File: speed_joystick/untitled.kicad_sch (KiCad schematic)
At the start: 48 parts

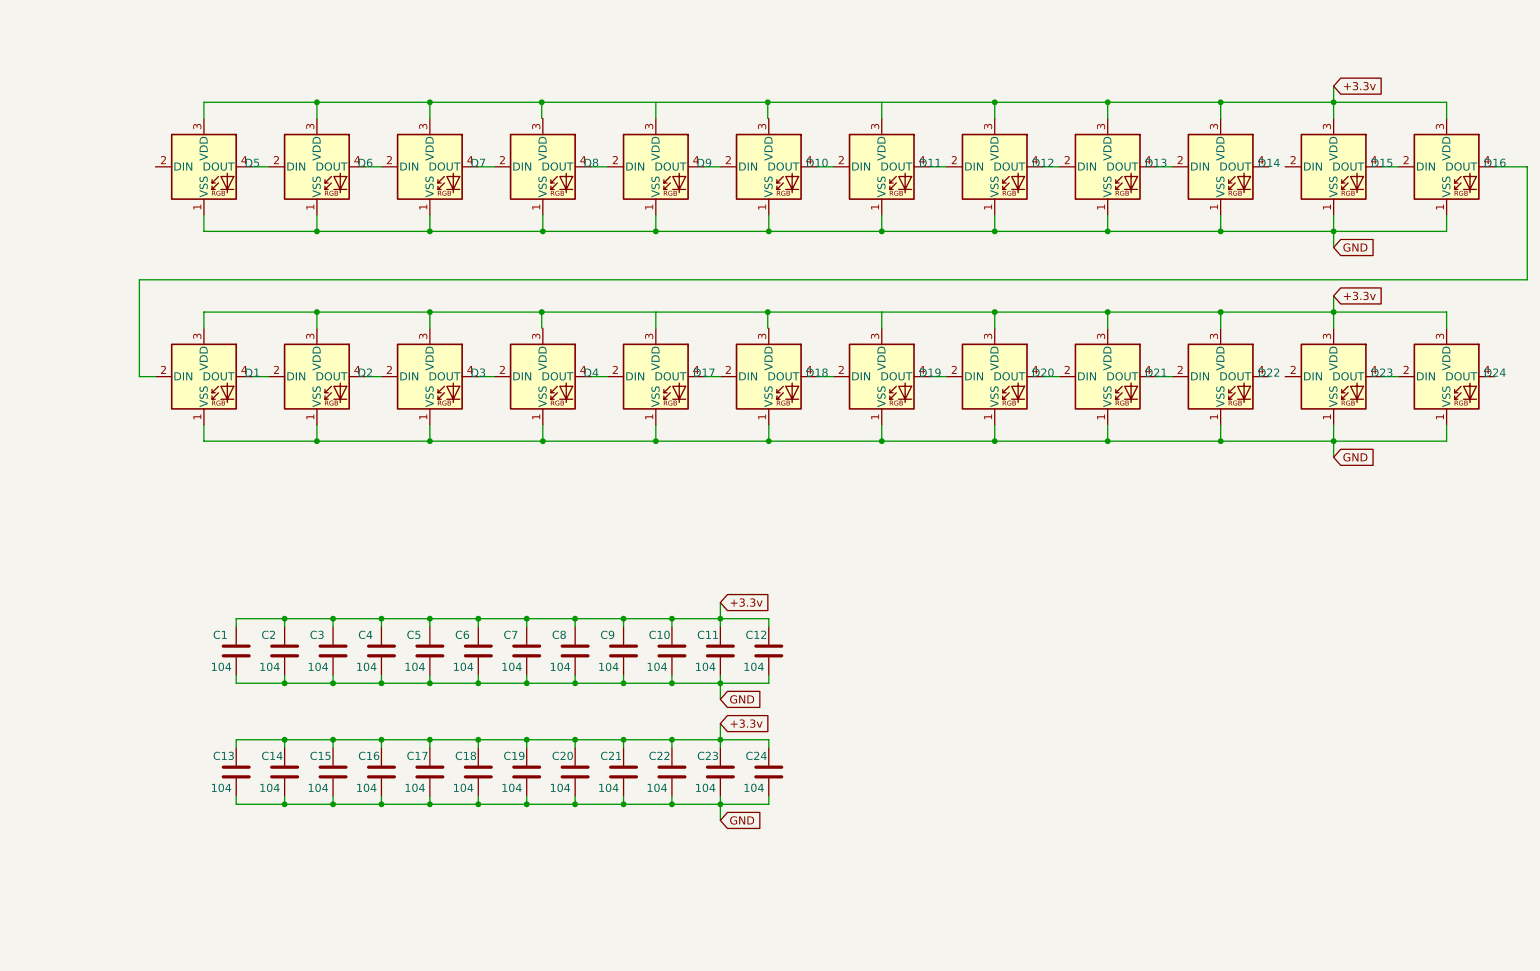
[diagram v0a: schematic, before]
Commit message: work on speed_joystick pcb
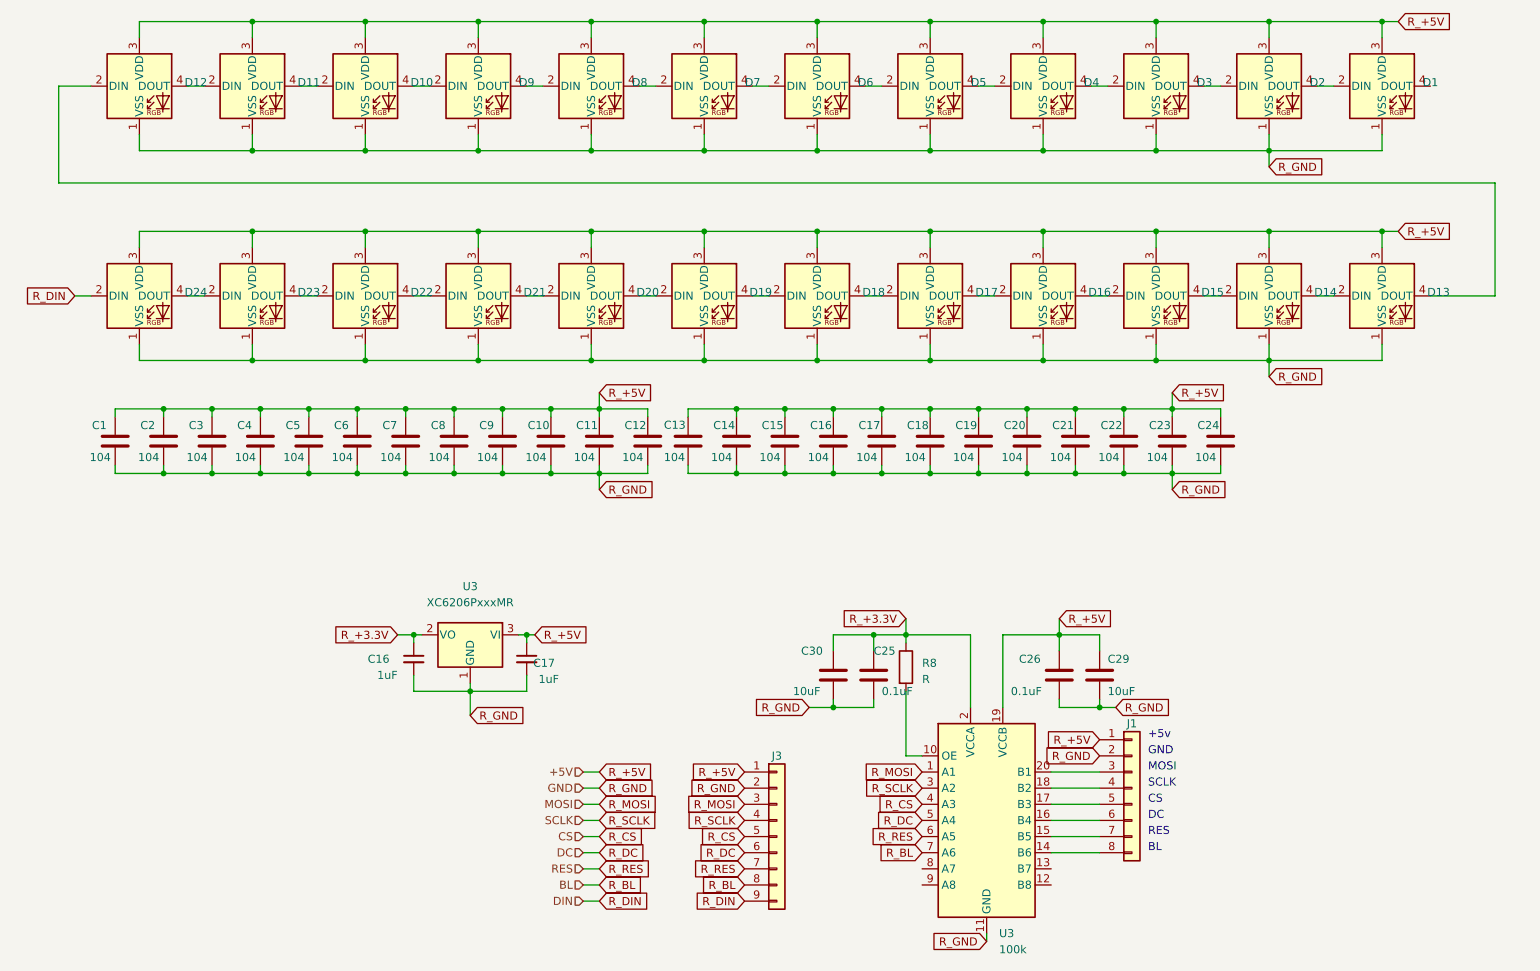
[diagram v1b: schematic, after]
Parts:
- added C16, C17: 1uF, Capacitor_SMD:C_0603_1608Metric, symbol Device:C_Small
- added C25, C26: 0.1uF, Capacitor_SMD:C_0603_1608Metric, symbol Device:C
- added C29, C30: 10uF, Capacitor_SMD:C_0603_1608Metric, symbol Device:C
- added J1: Conn_01x08, 8_hole:8_hole, symbol Connector_Generic:Conn_01x08
- added J3: Conn_01x09, Connector_PinSocket_2.54mm:PinSocket_1x09_P2.54mm_Vertical, symbol Connector_Generic:Conn_01x09
- added R8: R, Resistor_SMD:R_0805_2012Metric, symbol Device:R
- added U3: XC6206PxxxMR, Package_TO_SOT_SMD:SOT-23, symbol Regulator_Linear:XC6206PxxxMR
- added U3: 100k, Package_SO:TSSOP-20_4.4x6.5mm_P0.65mm, symbol Logic_LevelTranslator:TXS0108EPW
- D1: renamed from D16; footprint LED_SMD:LED_SK6812_PLCC4_5.0x5.0mm_P3.2mm -> LED_SMD:my_SK6812
- D10: renamed from D7; footprint LED_SMD:LED_SK6812_PLCC4_5.0x5.0mm_P3.2mm -> LED_SMD:my_SK6812
- D11: renamed from D6; footprint LED_SMD:LED_SK6812_PLCC4_5.0x5.0mm_P3.2mm -> LED_SMD:my_SK6812
- D12: renamed from D5; footprint LED_SMD:LED_SK6812_PLCC4_5.0x5.0mm_P3.2mm -> LED_SMD:my_SK6812
- D13: renamed from D24; footprint LED_SMD:LED_SK6812_PLCC4_5.0x5.0mm_P3.2mm -> LED_SMD:my_SK6812
- D14: renamed from D23; footprint LED_SMD:LED_SK6812_PLCC4_5.0x5.0mm_P3.2mm -> LED_SMD:my_SK6812
- D15: renamed from D22; footprint LED_SMD:LED_SK6812_PLCC4_5.0x5.0mm_P3.2mm -> LED_SMD:my_SK6812
- D16: renamed from D21; footprint LED_SMD:LED_SK6812_PLCC4_5.0x5.0mm_P3.2mm -> LED_SMD:my_SK6812
- D17: renamed from D20; footprint LED_SMD:LED_SK6812_PLCC4_5.0x5.0mm_P3.2mm -> LED_SMD:my_SK6812
- D18: renamed from D19; footprint LED_SMD:LED_SK6812_PLCC4_5.0x5.0mm_P3.2mm -> LED_SMD:my_SK6812
- D19: renamed from D18; footprint LED_SMD:LED_SK6812_PLCC4_5.0x5.0mm_P3.2mm -> LED_SMD:my_SK6812
- D2: renamed from D15; footprint LED_SMD:LED_SK6812_PLCC4_5.0x5.0mm_P3.2mm -> LED_SMD:my_SK6812
- D20: renamed from D17; footprint LED_SMD:LED_SK6812_PLCC4_5.0x5.0mm_P3.2mm -> LED_SMD:my_SK6812
- D21: renamed from D4; footprint LED_SMD:LED_SK6812_PLCC4_5.0x5.0mm_P3.2mm -> LED_SMD:my_SK6812
- D22: renamed from D3; footprint LED_SMD:LED_SK6812_PLCC4_5.0x5.0mm_P3.2mm -> LED_SMD:my_SK6812
- D23: renamed from D2; footprint LED_SMD:LED_SK6812_PLCC4_5.0x5.0mm_P3.2mm -> LED_SMD:my_SK6812
- D24: renamed from D1; footprint LED_SMD:LED_SK6812_PLCC4_5.0x5.0mm_P3.2mm -> LED_SMD:my_SK6812
- D3: renamed from D14; footprint LED_SMD:LED_SK6812_PLCC4_5.0x5.0mm_P3.2mm -> LED_SMD:my_SK6812
- D4: renamed from D13; footprint LED_SMD:LED_SK6812_PLCC4_5.0x5.0mm_P3.2mm -> LED_SMD:my_SK6812
- D5: renamed from D12; footprint LED_SMD:LED_SK6812_PLCC4_5.0x5.0mm_P3.2mm -> LED_SMD:my_SK6812
- D6: renamed from D11; footprint LED_SMD:LED_SK6812_PLCC4_5.0x5.0mm_P3.2mm -> LED_SMD:my_SK6812
- D7: renamed from D10; footprint LED_SMD:LED_SK6812_PLCC4_5.0x5.0mm_P3.2mm -> LED_SMD:my_SK6812
- D8: renamed from D9; footprint LED_SMD:LED_SK6812_PLCC4_5.0x5.0mm_P3.2mm -> LED_SMD:my_SK6812
- D9: renamed from D8; footprint LED_SMD:LED_SK6812_PLCC4_5.0x5.0mm_P3.2mm -> LED_SMD:my_SK6812
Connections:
- net +3.3v is gone; now on net R_+5V: C1.1, C10.1, C11.1, C12.1, C13.1, C14.1, C15.1, C16.1, C17.1, C18.1, C19.1, C2.1, C20.1, C21.1, C22.1, C23.1, C24.1, C3.1, C4.1, C5.1, C6.1, C7.1, C8.1, C9.1, D1.3 (VDD), D13.3 (VDD), D14.3 (VDD), D15.3 (VDD), D16.3 (VDD), D17.3 (VDD), D18.3 (VDD), D2.3 (VDD), D3.3 (VDD), D4.3 (VDD), D5.3 (VDD), D6.3 (VDD)
- net R_+5V: now reaches D19.3 (VDD)
- net R_+5V: now also D10.3 (VDD), D11.3 (VDD), D12.3 (VDD), D20.3 (VDD), D21.3 (VDD), D22.3 (VDD), D23.3 (VDD), D24.3 (VDD), D7.3 (VDD), D8.3 (VDD), D9.3 (VDD), C17.1, C26.1, C29.1, J1.1 (Pin_1), J3.1 (Pin_1), U3.19 (VCCB), U3.3 (VI)
- net at D1.4 (DOUT): no longer D24.2 (DIN)
- net at D13.4 (DOUT): now also D12.2 (DIN)
- net at D3.4 (DOUT): now also D2.2 (DIN)
- net at D15.4 (DOUT): now also D14.2 (DIN)
- net GND renamed R_GND
- net R_GND: now also C16.2, C17.2, C25.2, C26.2, C29.2, C30.2, J1.2 (Pin_2), J3.2 (Pin_2), U3.1 (GND), U3.11 (GND)
- new net: R8.2, U3.10 (OE)
- new net: J1.8 (Pin_8), U3.14 (B6)
- new net: J1.7 (Pin_7), U3.15 (B5)
- new net: J1.6 (Pin_6), U3.16 (B4)
- new net: J1.5 (Pin_5), U3.17 (B3)
- new net: J1.4 (Pin_4), U3.18 (B2)
- new net: J1.3 (Pin_3), U3.20 (B1)
- new net R_+3.3V: C16.1, C25.1, C30.1, R8.1, U3.2 (VCCA), U3.2 (VO)
- new net R_BL: J3.8 (Pin_8), U3.7 (A6)
- new net R_CS: J3.5 (Pin_5), U3.4 (A3)
- new net R_DC: J3.6 (Pin_6), U3.5 (A4)
- new net R_DIN: D24.2 (DIN), J3.9 (Pin_9)
- new net R_MOSI: J3.3 (Pin_3), U3.1 (A1)
- new net R_RES: J3.7 (Pin_7), U3.6 (A5)
- new net R_SCLK: J3.4 (Pin_4), U3.3 (A2)
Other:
- note added: "+5v"
- note added: "BL"
- note added: "CS"
- note added: "DC"
- note added: "GND"
- note added: "MOSI"
- note added: "RES"
- note added: "SCLK"
- moved on the sheet: C1, C10, C11, C12, C13, C14, C15, C16, C17, C18, C19, C2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
